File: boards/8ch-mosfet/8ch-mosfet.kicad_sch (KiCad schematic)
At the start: 7 parts, among them U1 ESP32-DEVKITC

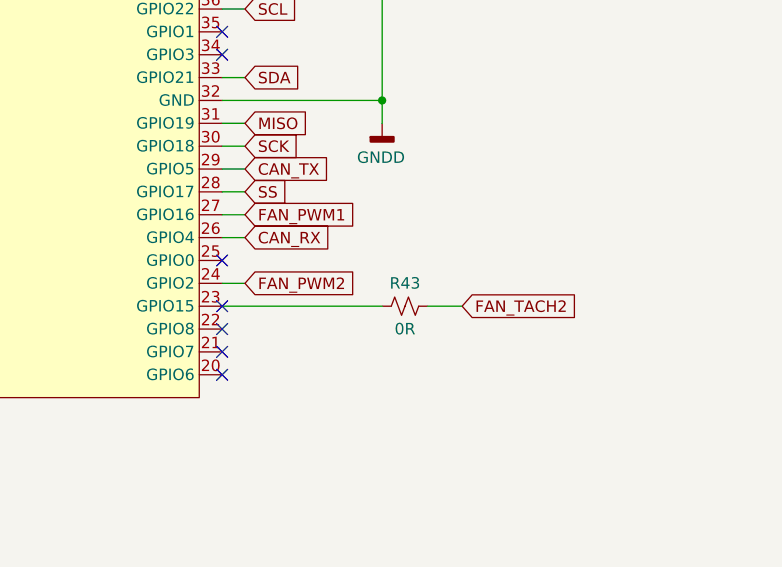
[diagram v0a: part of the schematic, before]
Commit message: reannotated
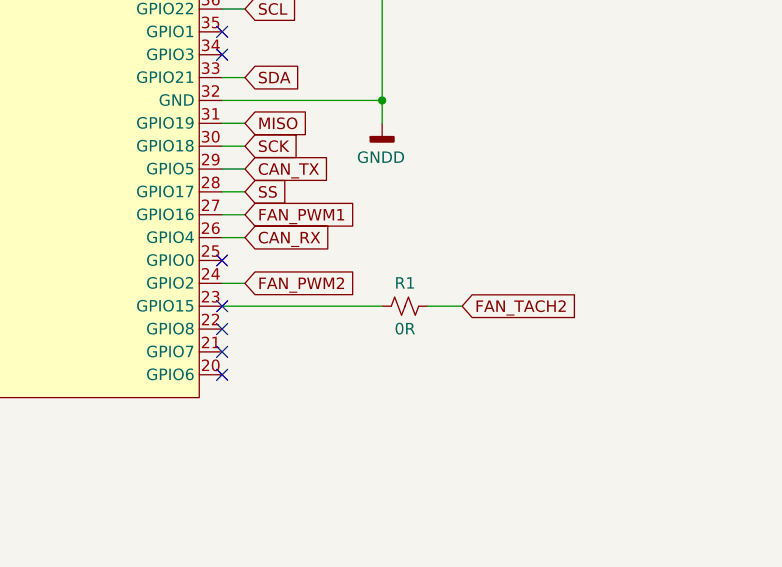
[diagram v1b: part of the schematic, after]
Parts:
- renumbered R43 to R1
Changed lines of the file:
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@@
   (symbol (lib_id "power:GNDD") (at 241.3 72.39 0) (unit 1)
     (in_bom yes) (on_board yes) (dnp no)
-    (property "Reference" "#PWR05" (at 241.3 78.74 0)
+    (property "Reference" "#PWR02" (at 241.3 78.74 0)
       (effects (font (size 1.27 1.27)) hide)
     )
@@
       (project "8ch-mosfet"
         (path "/c83c6236-96e9-46ad-9d7a-9e2efa4a7966"
-          (reference "#PWR05") (unit 1)
+          (reference "#PWR02") (unit 1)
         )
       )
@@
   (symbol (lib_id "Device:R_Small_US") (at 243.84 92.71 270) (unit 1)
     (in_bom yes) (on_board yes) (dnp no)
-    (property "Reference" "R43" (at 243.84 90.17 90)
+    (property "Reference" "R1" (at 243.84 90.17 90)
       (effects (font (size 1.27 1.27)))
     )
@@
       (project "8ch-mosfet"
         (path "/c83c6236-96e9-46ad-9d7a-9e2efa4a7966"
-          (reference "R43") (unit 1)
+          (reference "R1") (unit 1)
         )
         (path "/c83c6236-96e9-46ad-9d7a-9e2efa4a7966/0eec6767-666b-42c0-ba36-2a83c9caeade"
@@
   (symbol (lib_id "power:+3.3V") (at 181.61 49.53 0) (unit 1)
     (in_bom yes) (on_board yes) (dnp no) (fields_autoplaced)
-    (property "Reference" "#PWR02" (at 181.61 53.34 0)
+    (property "Reference" "#PWR01" (at 181.61 53.34 0)
       (effects (font (size 1.27 1.27)) hide)
     )
@@
       (project "8ch-mosfet"
         (path "/c83c6236-96e9-46ad-9d7a-9e2efa4a7966"
-          (reference "#PWR02") (unit 1)
+          (reference "#PWR01") (unit 1)
         )
       )
@@
   (symbol (lib_id "power:GNDD") (at 176.53 92.71 0) (unit 1)
     (in_bom yes) (on_board yes) (dnp no)
-    (property "Reference" "#PWR04" (at 176.53 99.06 0)
+    (property "Reference" "#PWR03" (at 176.53 99.06 0)
       (effects (font (size 1.27 1.27)) hide)
     )
@@
       (project "8ch-mosfet"
         (path "/c83c6236-96e9-46ad-9d7a-9e2efa4a7966"
-          (reference "#PWR04") (unit 1)
-        )
-      )
+          (reference "#PWR03") (unit 1)
+        )
+      )
